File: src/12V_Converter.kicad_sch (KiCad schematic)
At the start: 37 parts, among them M3 CSD19534Q5A, M4 NTMFS4D5N08XT1G, U2 LM5190RGYR_(20V-50V)

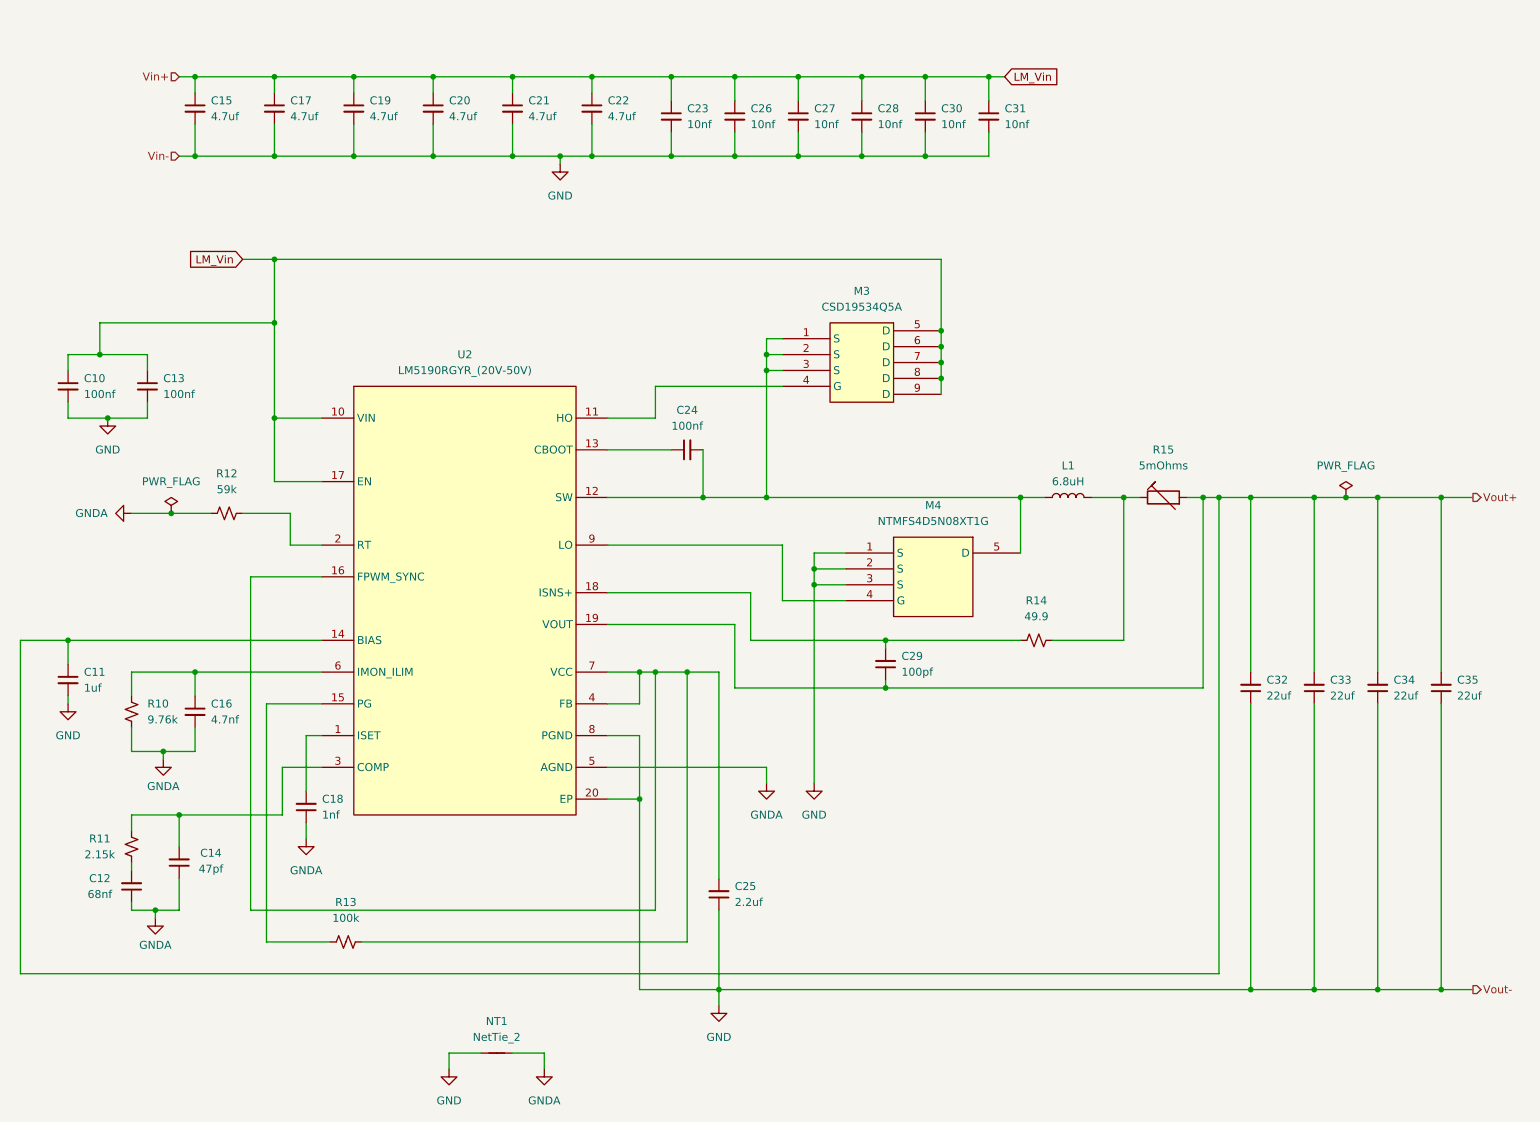
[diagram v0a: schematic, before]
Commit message: GG
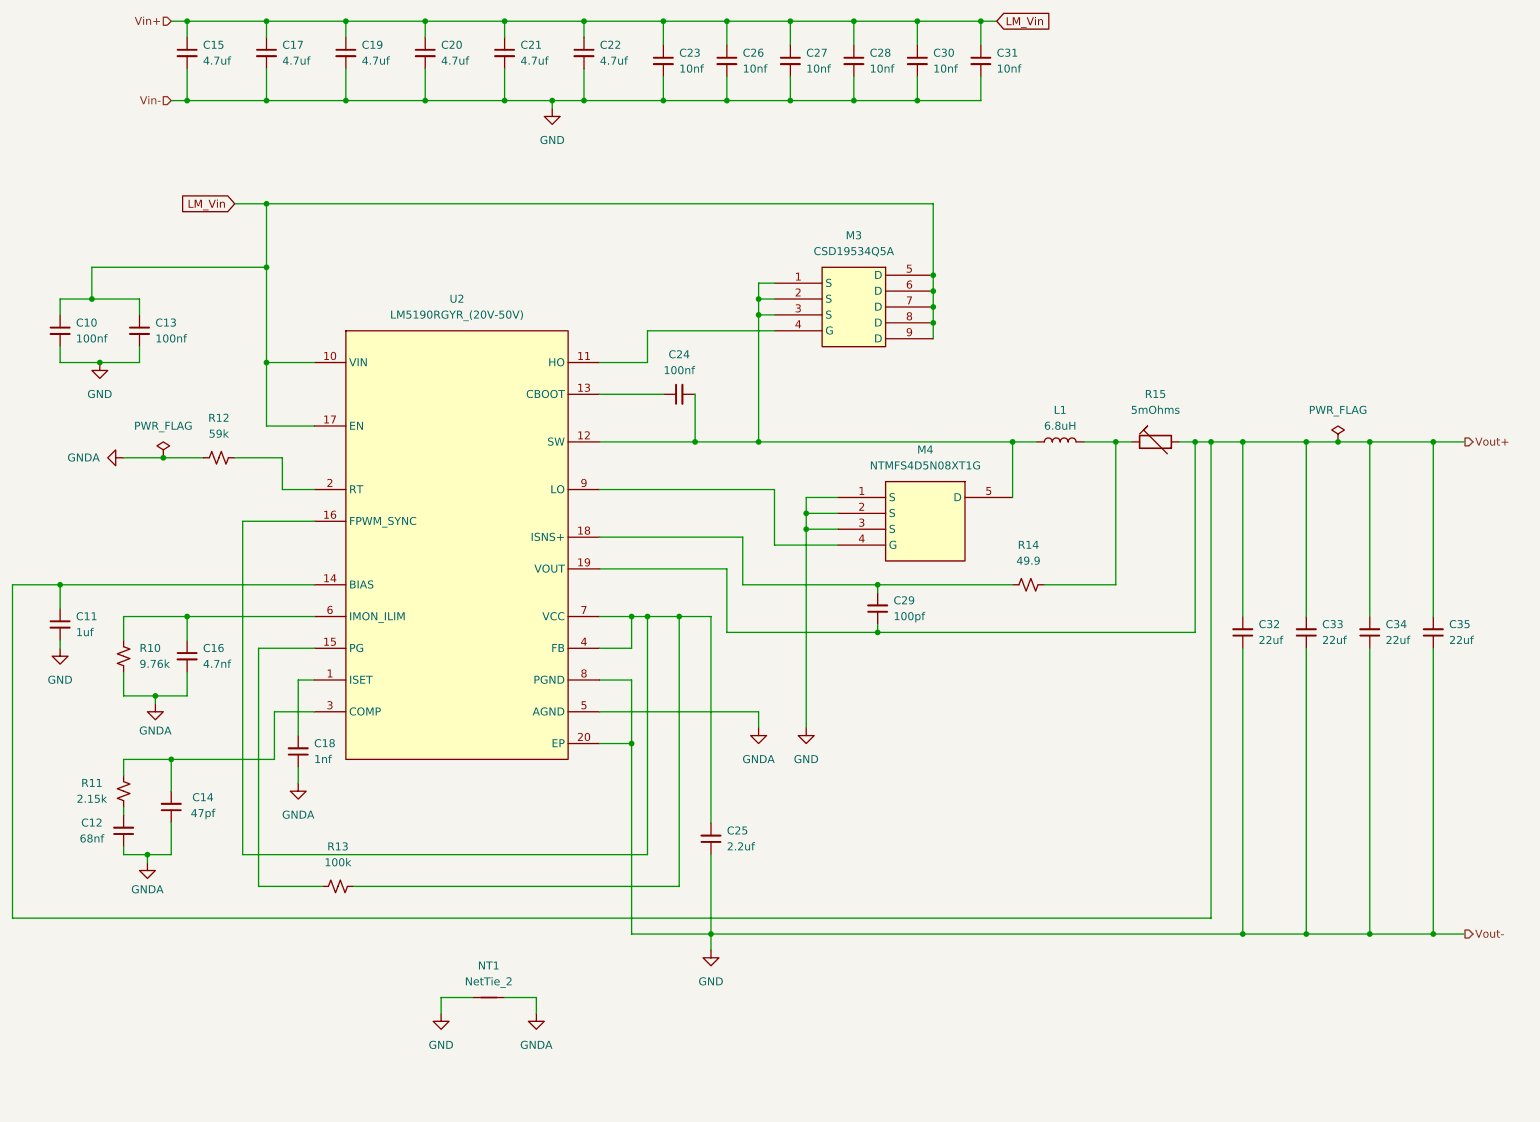
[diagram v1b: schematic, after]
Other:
- moved on the sheet: C10, C11, C12, C13, C14, C15, C16, C17, C18, C19, C20, C21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
